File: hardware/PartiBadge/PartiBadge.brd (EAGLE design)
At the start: 101.6 x 101.6 mm, 24 parts, among them J1 I2C, J2 Supply

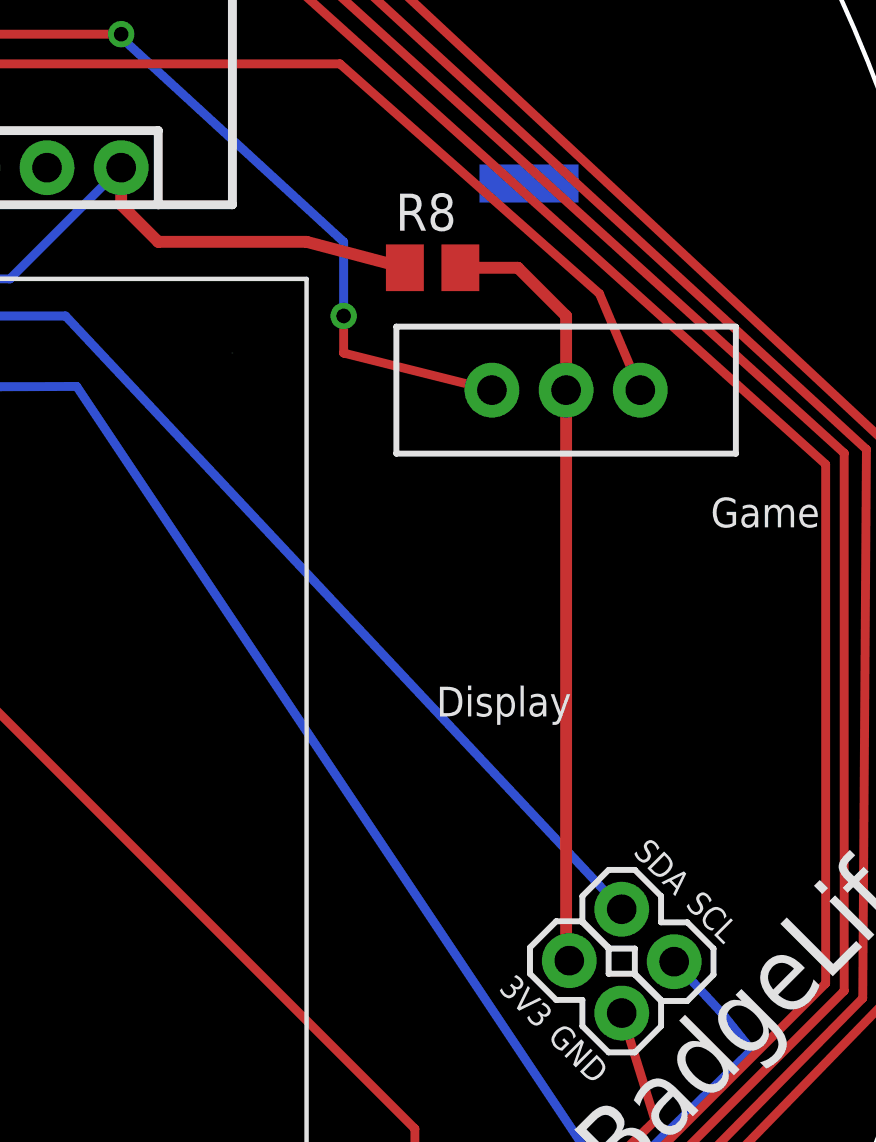
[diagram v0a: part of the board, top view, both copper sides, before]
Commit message: fix schematic and board with clr
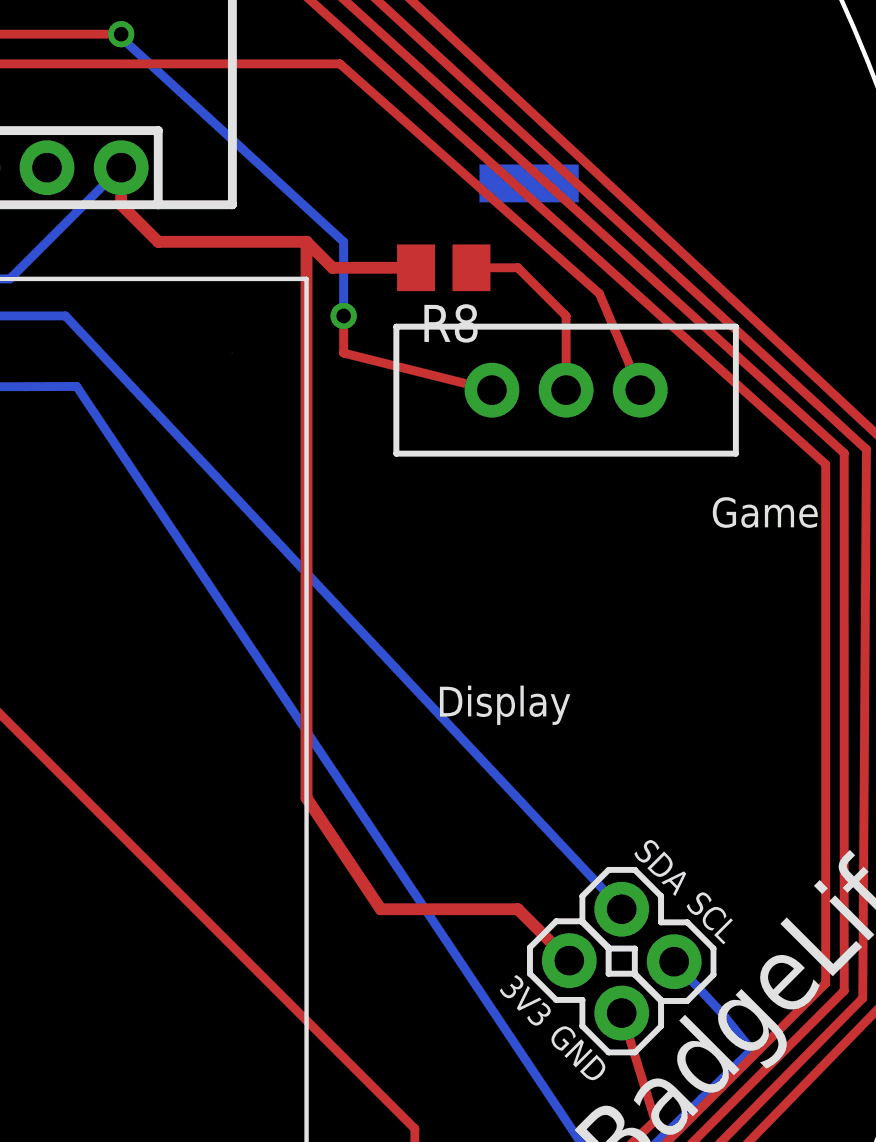
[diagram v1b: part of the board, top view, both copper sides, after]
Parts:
- moved R8 0.38 mm to (86.0, 69.0), turned to 180 degrees
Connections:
- new net N$14: R8.1, S5.2
- net 3V3: no longer R8.1, S5.2
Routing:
- net N$14: track 0.00 -> 6.46 mm
- net 3V3: track 134.6 -> 139.8 mm
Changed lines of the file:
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@@
 <attribute name="VERSION" value="v01" x="-1.27" y="10.16" size="1.778" layer="27" display="off"/>
 </element>
-<element name="R8" library="rcl" library_urn="urn:adsk.eagle:library:334" package="M0805" package3d_urn="urn:adsk.eagle:package:23556/1" value="100" x="85.598" y="68.961">
-<attribute name="SPICEPREFIX" value="R" x="85.598" y="68.961" size="1.778" layer="27" display="off"/>
+<element name="R8" library="rcl" library_urn="urn:adsk.eagle:library:334" package="M0805" package3d_urn="urn:adsk.eagle:package:23556/1" value="100" x="85.979" y="68.961" rot="R180">
+<attribute name="SPICEPREFIX" value="R" x="85.979" y="68.961" size="1.778" layer="27" rot="R180" display="off"/>
 </element>
 </elements>
@@
 <wire x1="76.2" y1="69.85" x2="81.28" y2="69.85" width="0.4064" layer="1"/>
 <contactref element="R8" pad="2"/>
-<contactref element="S5" pad="2"/>
-<contactref element="R8" pad="1"/>
-<wire x1="81.28" y1="69.85" x2="84.648" y2="68.961" width="0.4064" layer="1"/>
-<wire x1="86.548" y1="68.961" x2="88.519" y2="68.961" width="0.4064" layer="1"/>
-<wire x1="88.519" y1="68.961" x2="90.17" y2="67.31" width="0.4064" layer="1"/>
-<wire x1="90.17" y1="67.31" x2="90.17" y2="64.77" width="0.4064" layer="1"/>
-<wire x1="90.17" y1="64.77" x2="90.17" y2="45.338996875" width="0.4064" layer="1"/>
-<wire x1="84.648" y1="68.961" x2="86.548" y2="68.961" width="0" layer="19" extent="1-1"/>
+<wire x1="82.169" y1="68.961" x2="81.28" y2="69.85" width="0.4064" layer="1"/>
+<wire x1="85.029" y1="68.961" x2="82.169" y2="68.961" width="0.4064" layer="1"/>
+<wire x1="81.28" y1="69.85" x2="81.28" y2="50.8" width="0.4064" layer="1"/>
+<wire x1="81.28" y1="50.8" x2="83.82" y2="46.99" width="0.4064" layer="1"/>
+<wire x1="88.518996875" y1="46.99" x2="90.278946875" y2="45.23005" width="0.4064" layer="1"/>
+<wire x1="83.82" y1="46.99" x2="88.518996875" y2="46.99" width="0.4064" layer="1"/>
 </signal>
 <signal name="N$4">
@@
 <wire x1="10.16" y1="68.58" x2="11.43" y2="69.85" width="0.3048" layer="1"/>
 </signal>
+<signal name="N$14">
+<contactref element="S5" pad="2"/>
+<contactref element="R8" pad="1"/>
+<wire x1="90.17" y1="64.77" x2="90.17" y2="67.31" width="0.3048" layer="1"/>
+<wire x1="90.17" y1="67.31" x2="88.519" y2="68.961" width="0.3048" layer="1"/>
+<wire x1="88.519" y1="68.961" x2="86.929" y2="68.961" width="0.3048" layer="1"/>
+</signal>
 </signals>

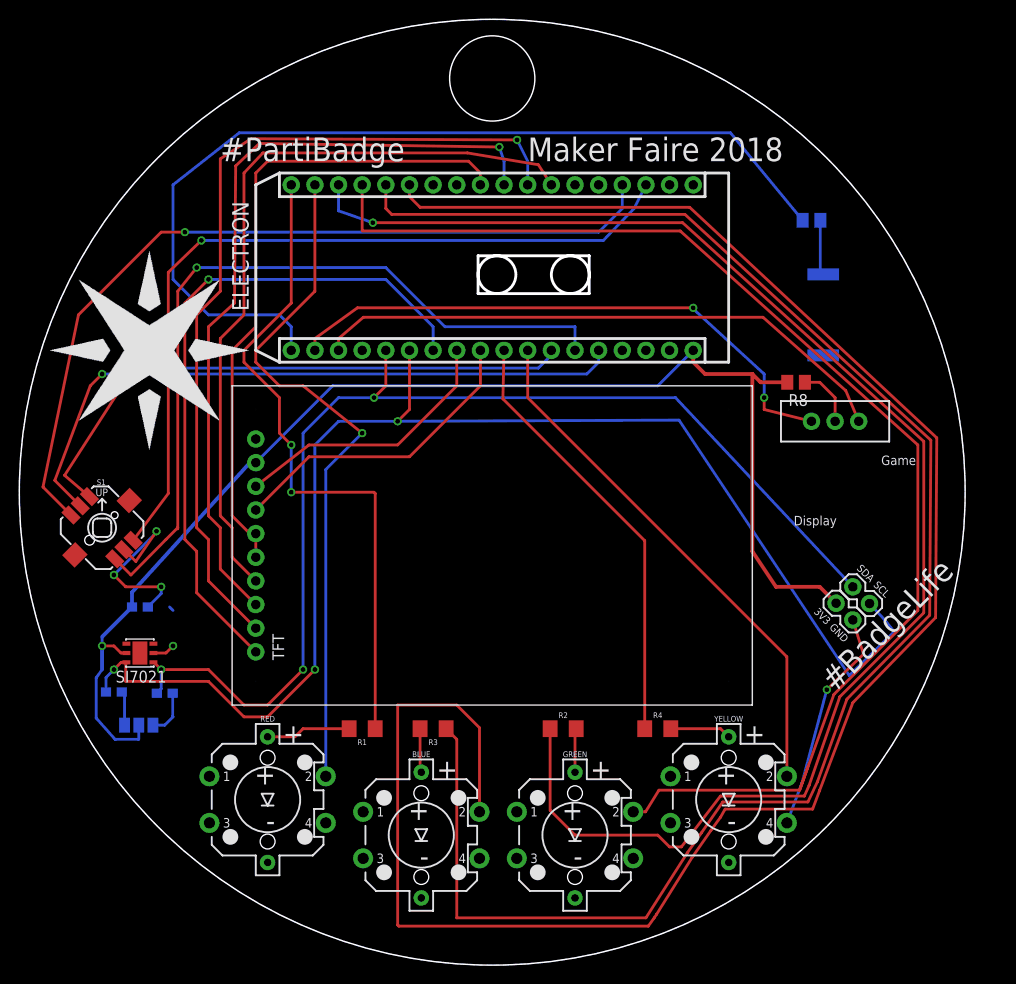
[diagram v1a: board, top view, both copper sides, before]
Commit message: cleaning up routes
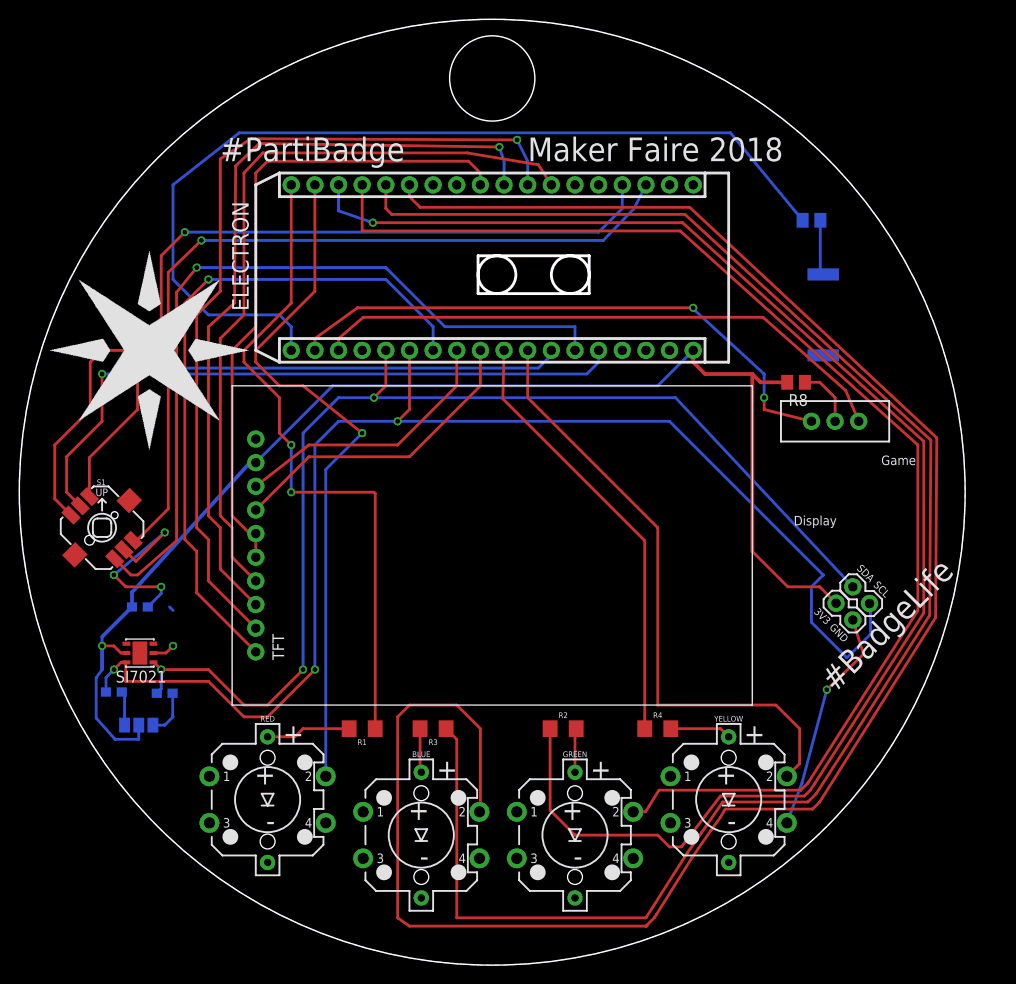
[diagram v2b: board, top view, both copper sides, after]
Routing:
- net BUTTON_YELLOW: track 57.3 -> 65.9 mm
- net SCL: track 146.7 -> 143.2 mm
- net N$6: track 136.8 -> 133.6 mm
- net LEFT: track 88.8 -> 91.2 mm
- net N$9: track 206.5 -> 204.8 mm
- net UP: track 63.8 -> 62.4 mm
- net GND: track 47.9 -> 48.9 mm
- net LED_GREEN: track 157.8 -> 157.3 mm
- net RIGHT: track 85.8 -> 86.3 mm
- net LED_BLUE: track 179.3 -> 178.8 mm
